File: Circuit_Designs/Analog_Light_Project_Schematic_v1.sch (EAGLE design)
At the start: 19 parts, among them IC2 4026N, T1 2N2222, T2 2N2222, T3 2N2222

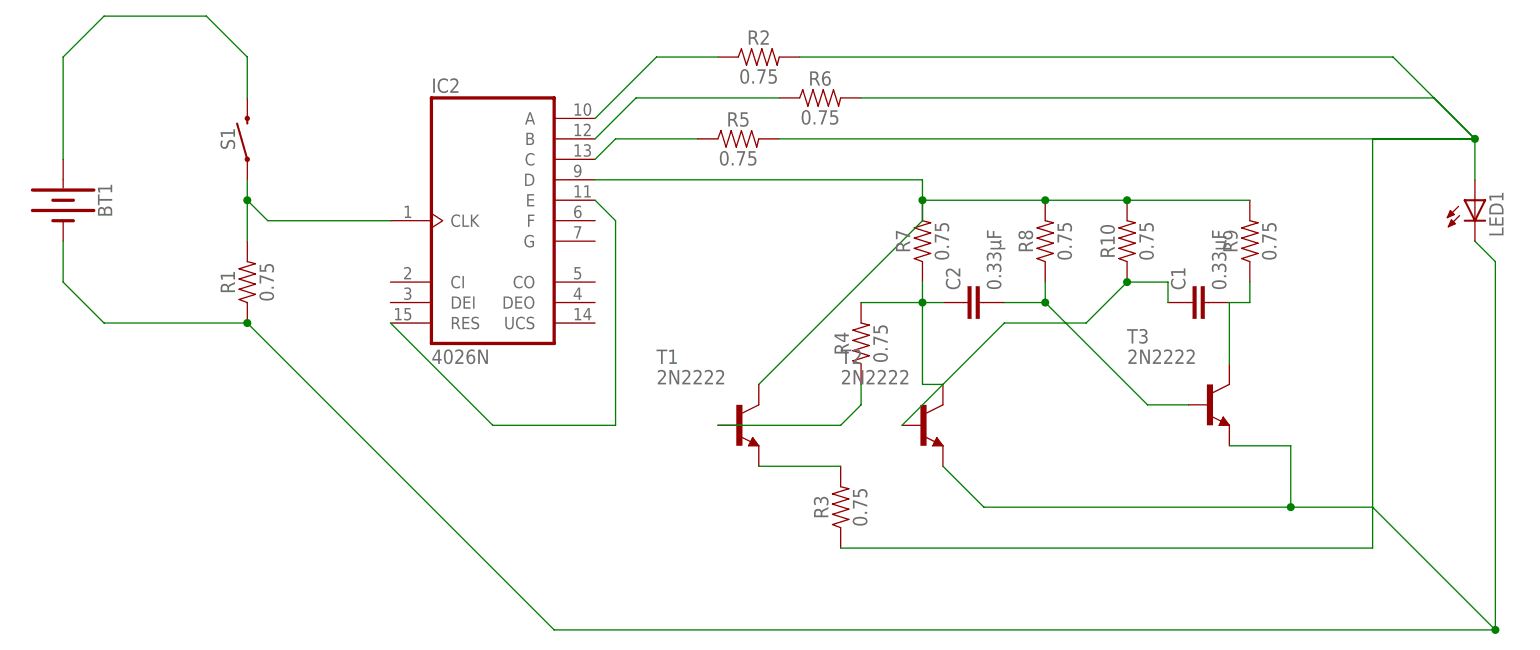
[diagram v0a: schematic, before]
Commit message: Add files via upload
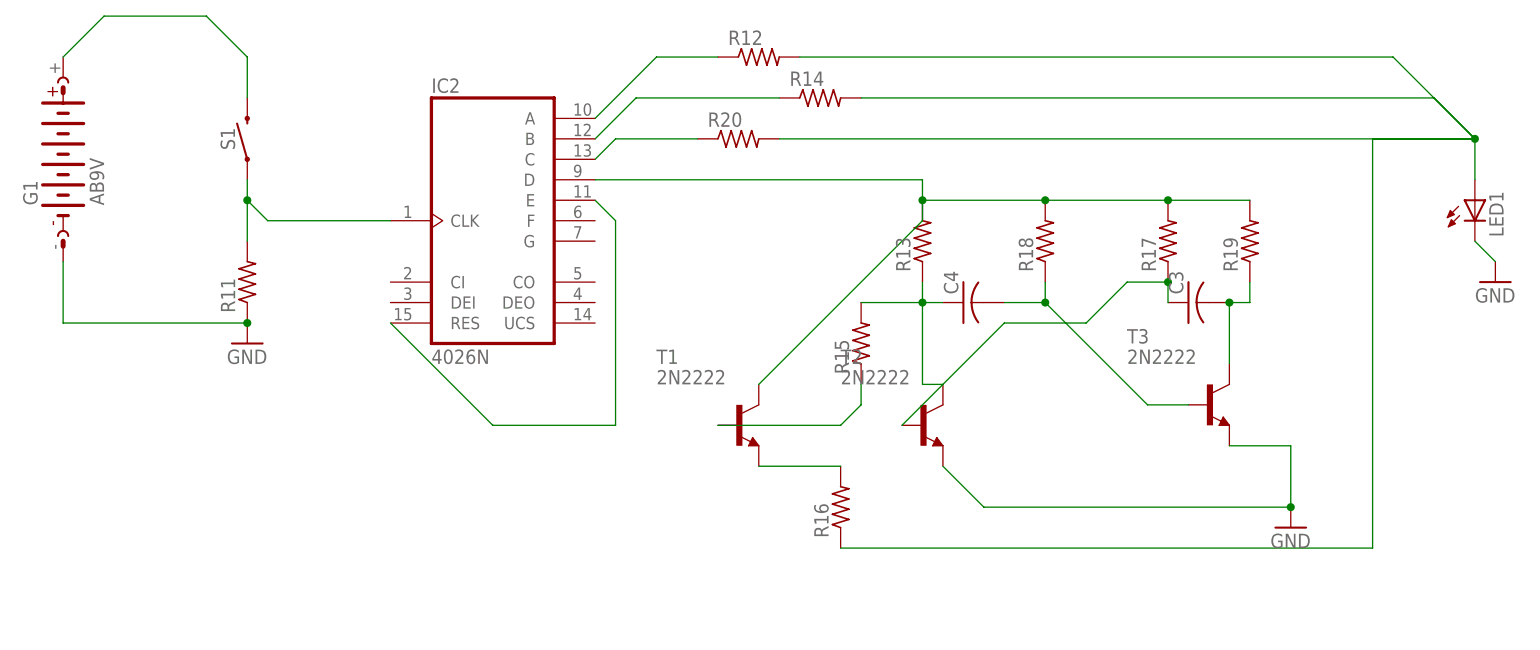
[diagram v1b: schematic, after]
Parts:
- removed BT1: (no value), SparkFun-Batteries:BATTERY-9V
- removed C1, C2: 0.33µF, SparkFun-Capacitors:0.33UF/330NF-0805-50V-10%
- removed R1, R10, R2, R3, R4, R5, R6, R7, R8, R9: 0.75, SparkFun-Resistors:0.75OHM-0805-1/4W-1%
- added C3, C4: (no value), adafruit:C-USC0805
- added G1: AB9V, battery:AB9V
- added R11, R12, R13, R14, R15, R16, R17, R18, R19, R20: (no value), adafruit:R-US_M0805
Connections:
- removed net N$6: BT1.-, LED1.C, R1.1, T2.E, T3.E
- new net GND: G1.-, LED1.C, R11.1, T2.E, T3.E
- net N$1: now also R13.2, R17.2, R18.2, R19.2; no longer R10.2, R7.2, R8.2, R9.2
- net N$10: now also R12.1; no longer R2.1
- net N$11: now also R14.1; no longer R6.1
- net N$12: now also R20.1; no longer R5.1
- net N$14: now also G1.+; no longer BT1.+
- net N$15: now also R11.2; no longer R1.2
- net N$2: now also C4.1, R13.1, R15.2; no longer C2.1, R4.2, R7.1
- net N$3: now also C4.2, R18.1; no longer C2.2, R8.1
- net N$4: now also C3.1, R17.1; no longer C1.1, R10.1
- net N$5: now also C3.2, R19.1; no longer C1.2, R9.1
- net N$7: now also R15.1; no longer R4.1
- net N$8: now also R16.2; no longer R3.2
- net N$9: now also R12.2, R14.2, R16.1, R20.2; no longer R2.2, R3.1, R5.2, R6.2
